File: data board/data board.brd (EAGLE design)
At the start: 47.6 x 28 mm, 43 parts, among them IC1 93LC56B, IC2 FT232HQ, U1 CJT1117-5.0-SOT223, X3 HUSB238, X6 USBC, Y1 12MHz

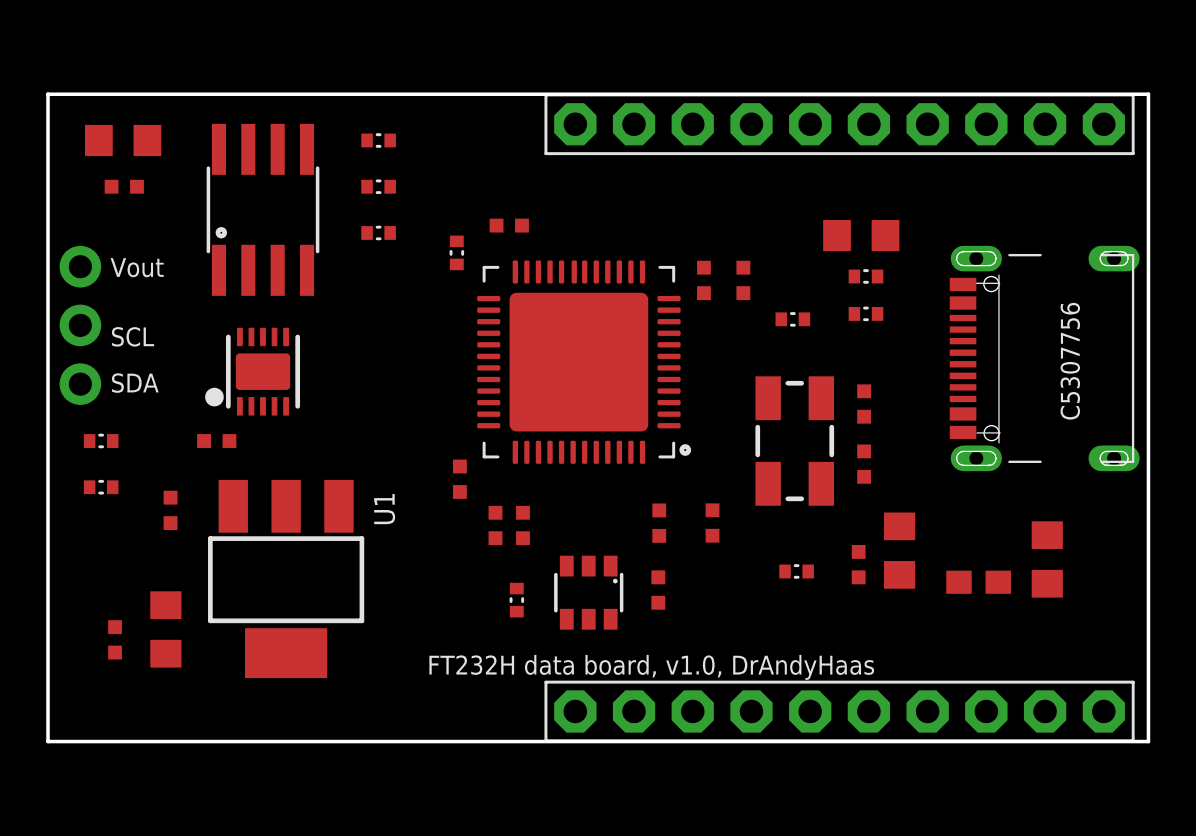
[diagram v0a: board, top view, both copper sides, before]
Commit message: v1.1
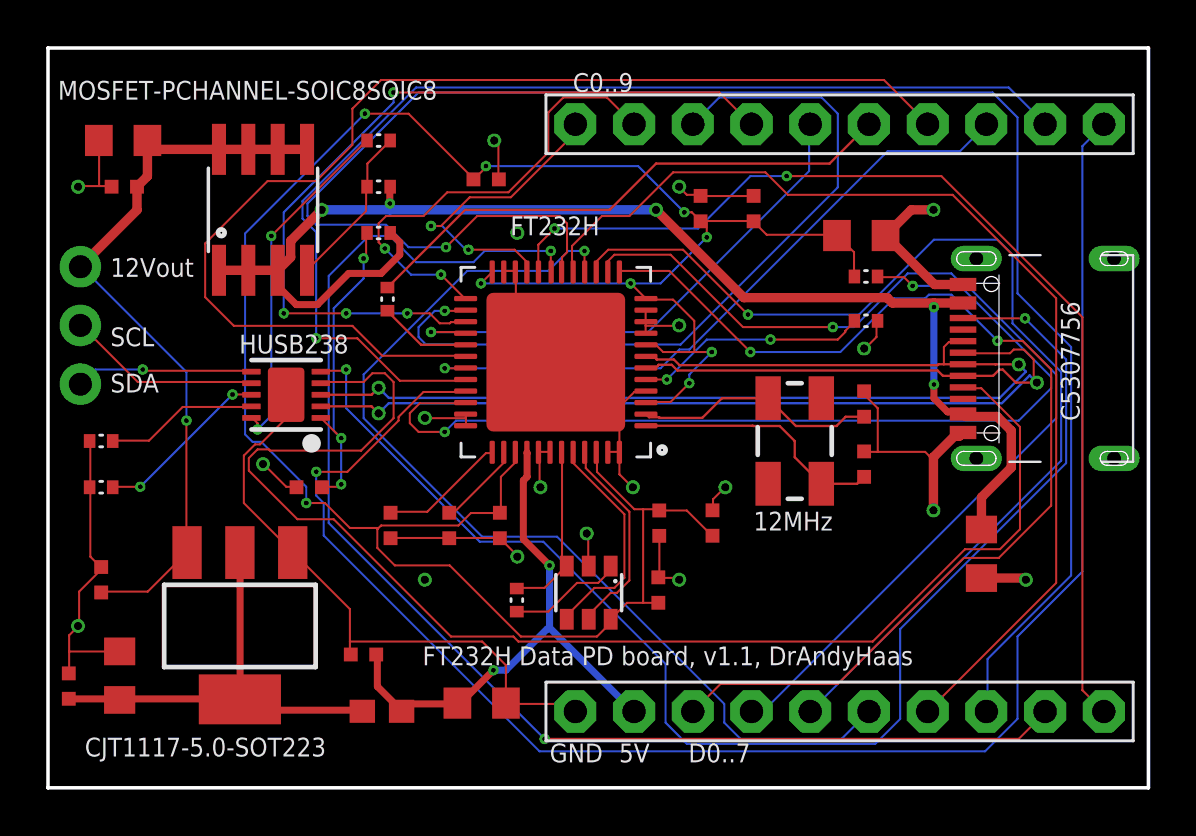
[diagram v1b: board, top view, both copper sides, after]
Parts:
- removed R3, R5: 5.1k, FlashPCB_Resistors:RES-0402
- moved FB1 26.4 mm to (0.15, -4.69), turned to 0 degrees
- moved C6 21.8 mm to (-0.65, -2.23), turned to 0 degrees
- moved C13 19.3 mm to (4.41, -4.34), turned to 180 degrees
- moved C16 4.47 mm to (-3.00, 5.00)
- moved C21 4.24 mm to (-12.0, 1.00)
- moved C4 3.61 mm to (0.52, 3.35)
- moved R6 3.61 mm to (0.38, 13.1)
- moved C10 3.14 mm to (16.2, 17.1), turned to 270 degrees
- moved C5 3.11 mm to (13.9, 17.1), turned to 270 degrees
- moved C7 2.87 mm to (26.1, 2.17), turned to 90 degrees
- moved C19 2.83 mm to (-11.2, -3.20)
- moved C20 2.83 mm to (-13.4, -3.60)
- moved U1 2.83 mm to (-6.00, -1.00)
- moved C9 2.24 mm to (4.65, 18.3)
- moved C2 2.00 mm to (3.06, 3.35)
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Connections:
- new net 5VD: C19.2, C20.2, FB1.1, U1.2, U1.TER
- net 5V: no longer C19.2, C20.2, U1.2, U1.TER
- net CC1: no longer R5.P$2
- net CC2: no longer R3.P$2
- net GND: no longer R3.P$1, R5.P$1
- net VBUS: no longer FB1.1
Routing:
- net VCC3V3: track 0.00 -> 107.9 mm, vias 0 -> 9
- net GND: track 0.00 -> 102.3 mm, vias 0 -> 19
- net D5: track 0.00 -> 76.6 mm, vias 0 -> 1
- net C9: track 0.00 -> 72.6 mm, vias 0 -> 1
- net CC1: track 0.00 -> 58.7 mm
- net CC2: track 0.00 -> 58.4 mm, vias 0 -> 2
- net D6: track 0.00 -> 58.0 mm, vias 0 -> 2
- net VBUS: track 0.00 -> 57.5 mm, vias 0 -> 5
- net D_P: track 0.00 -> 53.8 mm, vias 0 -> 2
- net C6: track 0.00 -> 50.6 mm
- net D_N: track 0.00 -> 49.7 mm, vias 0 -> 2
- net C8: track 0.00 -> 48.3 mm, vias 0 -> 1
- net D0: track 0.00 -> 47.6 mm, vias 0 -> 2
- net D2: track 0.00 -> 46.6 mm, vias 0 -> 1
- net D7: track 0.00 -> 45.9 mm, vias 0 -> 2
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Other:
- board size 47.6 x 28 mm -> 47.6 x 32 mm
- board text added: "12Vout"
- board text added: "5V"
- board text added: "C0..9"
- board text added: "D0..7"
- board text added: "FT232H"
- board text added: "FT232H Data PD board, v1.1, DrAndyHaas"
- board text added: "GND"
- board text removed: "FT232H data board, v1.0, DrAndyHaas"
- board text removed: "Vout"

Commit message: Revert "v1.1"
This reverts commit 3ea246ff6ce0038198bb0009f8cc6fa5045fb056.
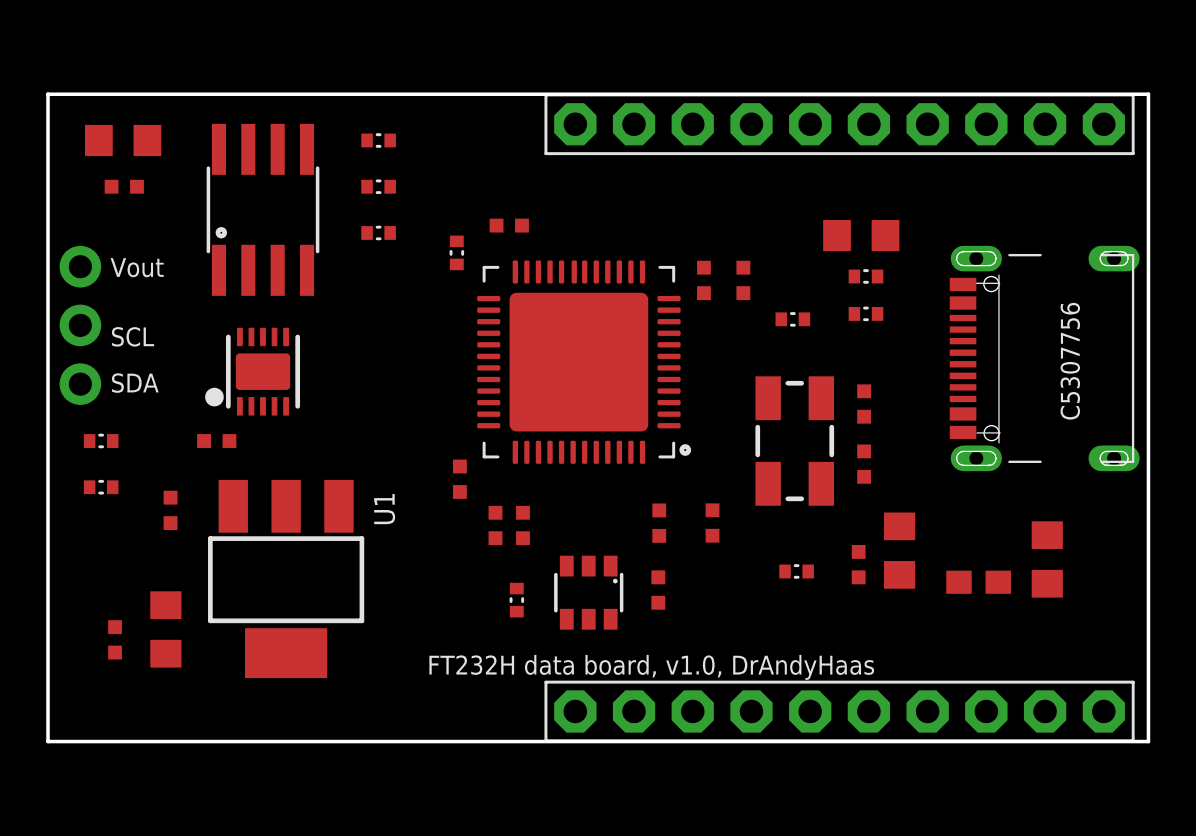
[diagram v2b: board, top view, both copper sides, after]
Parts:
- added R3, R5: 5.1k, FlashPCB_Resistors:RES-0402
- moved FB1 26.4 mm to (26.0, 0.89), turned to 180 degrees
- moved C6 21.8 mm to (20.8, 1.65), turned to 270 degrees
- moved C13 19.3 mm to (22.5, 2.21), turned to 270 degrees
- moved C16 4.47 mm to (-7.00, 7.00)
- moved C21 4.24 mm to (-9.00, 4.00)
- moved C4 3.61 mm to (3.52, 5.35)
- moved R6 3.61 mm to (3.38, 15.1)
- moved C10 3.14 mm to (15.8, 13.9), turned to 90 degrees
- moved C5 3.11 mm to (14.1, 13.9), turned to 90 degrees
- moved C7 2.87 mm to (28.9, 1.83), turned to 270 degrees
- moved C19 2.83 mm to (-9.20, -1.20)
- moved C20 2.83 mm to (-11.4, -1.60)
- moved U1 2.83 mm to (-4.00, 1.00)
- moved C9 2.24 mm to (5.65, 16.3)
- moved C2 2.00 mm to (5.06, 3.35)
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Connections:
- removed net 5VD: C19.2, C20.2, FB1.1, U1.2, U1.TER
- net 5V: now also C19.2, C20.2, U1.2, U1.TER
- net CC1: now also R5.P$2
- net CC2: now also R3.P$2
- net GND: now also R3.P$1, R5.P$1
- net VBUS: now also FB1.1
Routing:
- net VCC3V3: track 107.9 -> 0.00 mm, vias 9 -> 0
- net GND: track 102.3 -> 0.00 mm, vias 19 -> 0
- net D5: track 76.6 -> 0.00 mm, vias 1 -> 0
- net C9: track 72.6 -> 0.00 mm, vias 1 -> 0
- net CC1: track 58.7 -> 0.00 mm
- net CC2: track 58.4 -> 0.00 mm, vias 2 -> 0
- net D6: track 58.0 -> 0.00 mm, vias 2 -> 0
- net VBUS: track 57.5 -> 0.00 mm, vias 5 -> 0
- net D_P: track 53.8 -> 0.00 mm, vias 2 -> 0
- net C6: track 50.6 -> 0.00 mm
- net D_N: track 49.7 -> 0.00 mm, vias 2 -> 0
- net C8: track 48.3 -> 0.00 mm, vias 1 -> 0
- net D0: track 47.6 -> 0.00 mm, vias 2 -> 0
- net D2: track 46.6 -> 0.00 mm, vias 1 -> 0
- net D7: track 45.9 -> 0.00 mm, vias 2 -> 0
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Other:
- board size 47.6 x 32 mm -> 47.6 x 28 mm
- board text added: "FT232H data board, v1.0, DrAndyHaas"
- board text added: "Vout"
- board text removed: "12Vout"
- board text removed: "5V"
- board text removed: "C0..9"
- board text removed: "D0..7"
- board text removed: "FT232H"
- board text removed: "FT232H Data PD board, v1.1, DrAndyHaas"
- board text removed: "GND"
